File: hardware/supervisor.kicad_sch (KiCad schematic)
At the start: 39 parts, among them U5 STM32L4P5RET6, U6 MCP2562-H-SN, Y1 Crystal_GND24

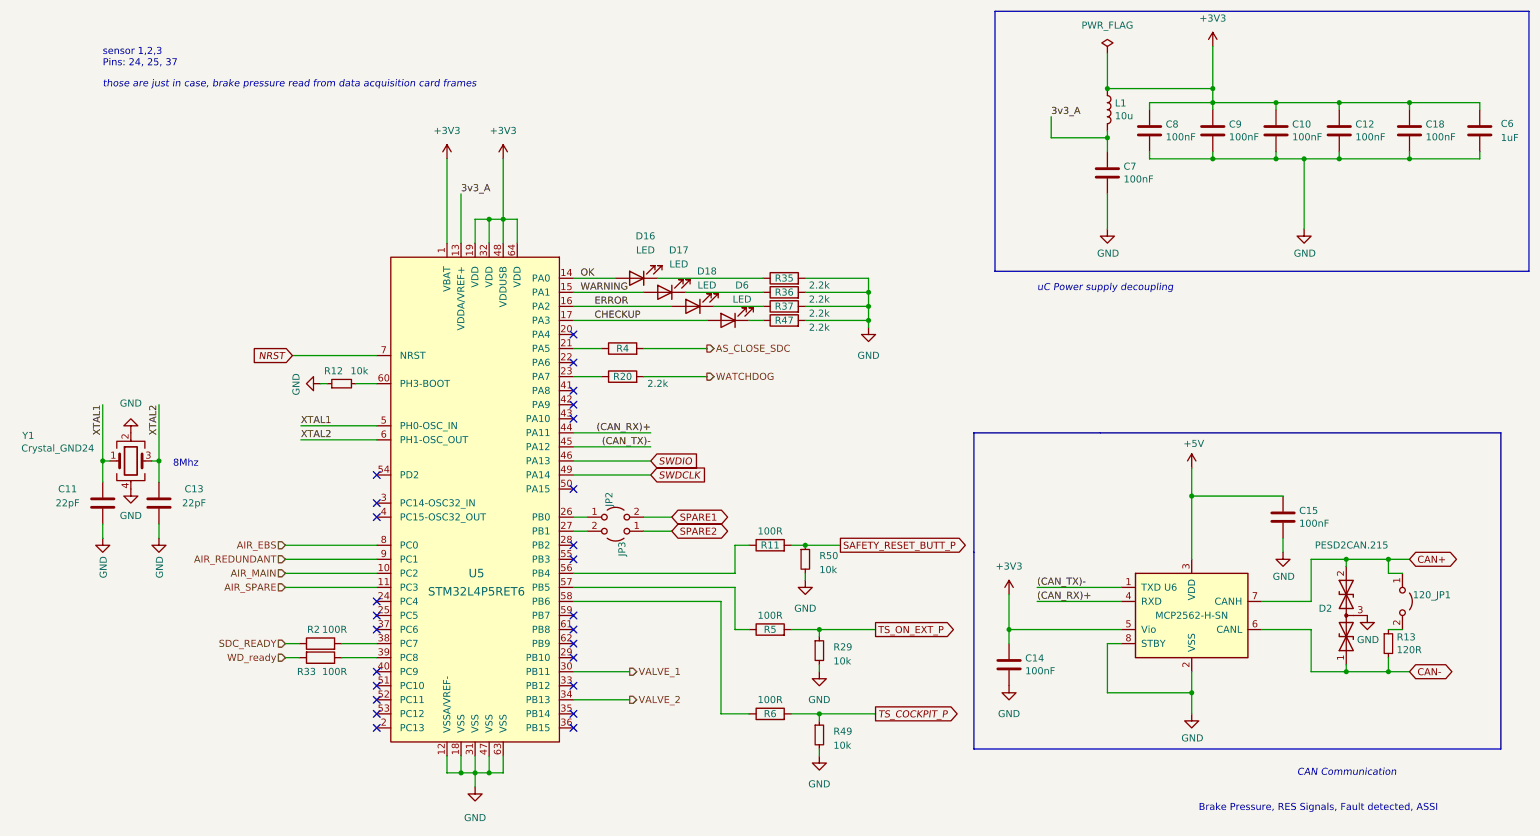
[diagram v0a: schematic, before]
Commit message: WIP 1.1 routing
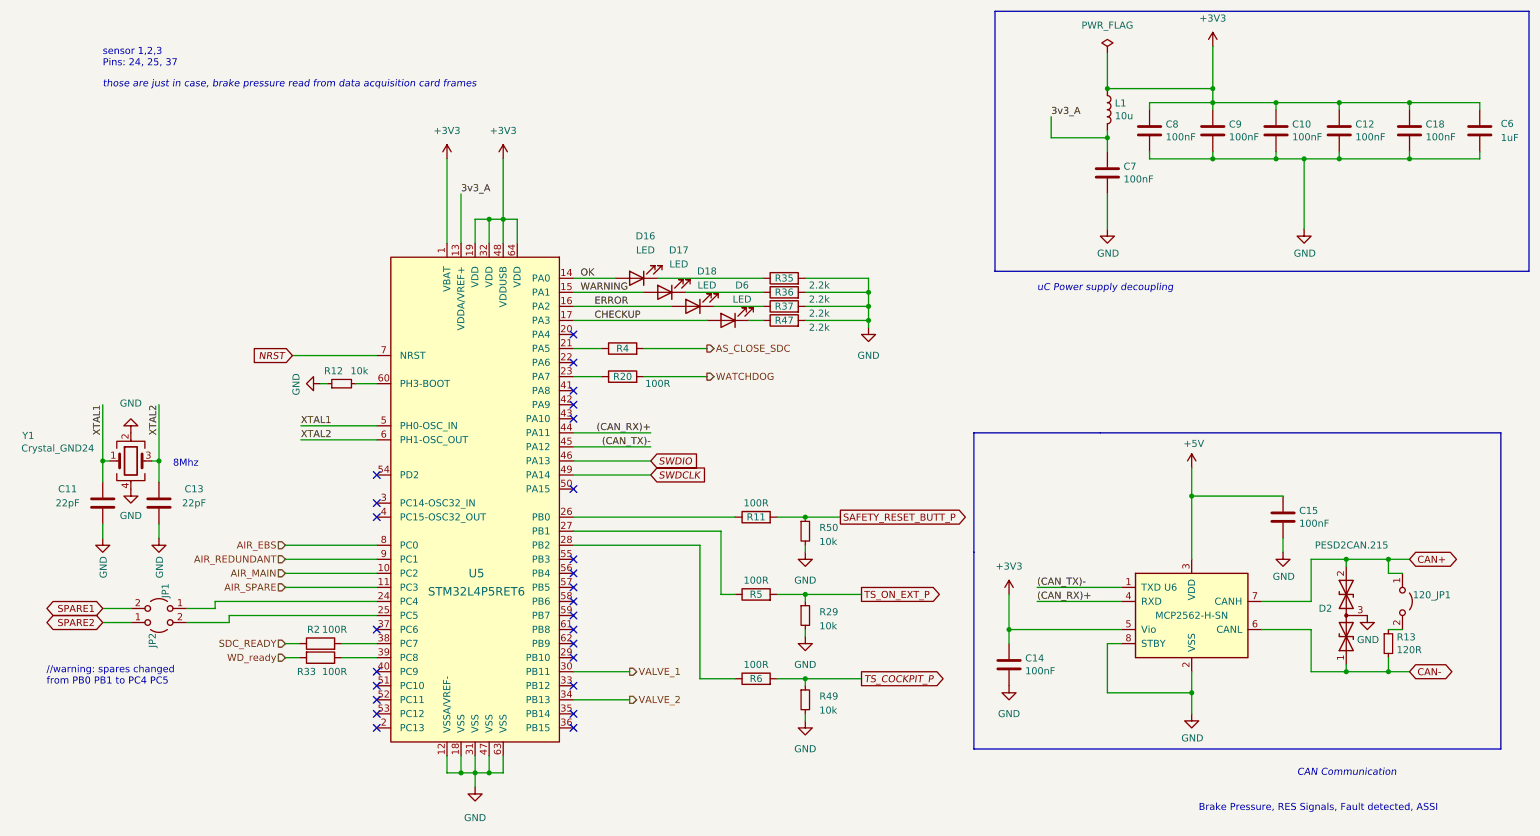
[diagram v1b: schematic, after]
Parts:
- removed JP3: Jumper_NC_Small, Jumper:SolderJumper-2_P1.3mm_Open_RoundedPad1.0x1.5mm, symbol Jumper:Jumper_2_Open
- added JP1: Jumper_NC_Small, Jumper:SolderJumper-2_P1.3mm_Open_RoundedPad1.0x1.5mm, symbol Jumper:Jumper_2_Open
- R20, R4: value 2.2k -> 100R
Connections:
- net SPARE1: now also JP1.2 (B); no longer JP2.2 (B)
- net SPARE2: now also JP2.1 (A)
- net at U5.27 (PB1): now also R5.1
- net at U5.57 (PB5): no longer R5.1
- net at U5.24 (PC4): now also JP1.1 (A)
- net at U5.25 (PC5): now also JP2.2 (B)
- net at U5.26 (PB0): now also R11.1; no longer JP2.1 (A)
- net at U5.28 (PB2): now also R6.1
- net at U5.56 (PB4): no longer R11.1
- net at U5.58 (PB6): no longer R6.1
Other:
- note added: "//warning: spares changed from PB0 PB1 to PC4 PC5"
- moved on the sheet: R11, R29, R49, R5, R50, R6
